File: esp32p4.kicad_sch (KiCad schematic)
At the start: 51 parts, among them U13 W25Q128JVS, U3 TLV62569DBV, U8 ESP32P4-REV0, Y3 40MHz

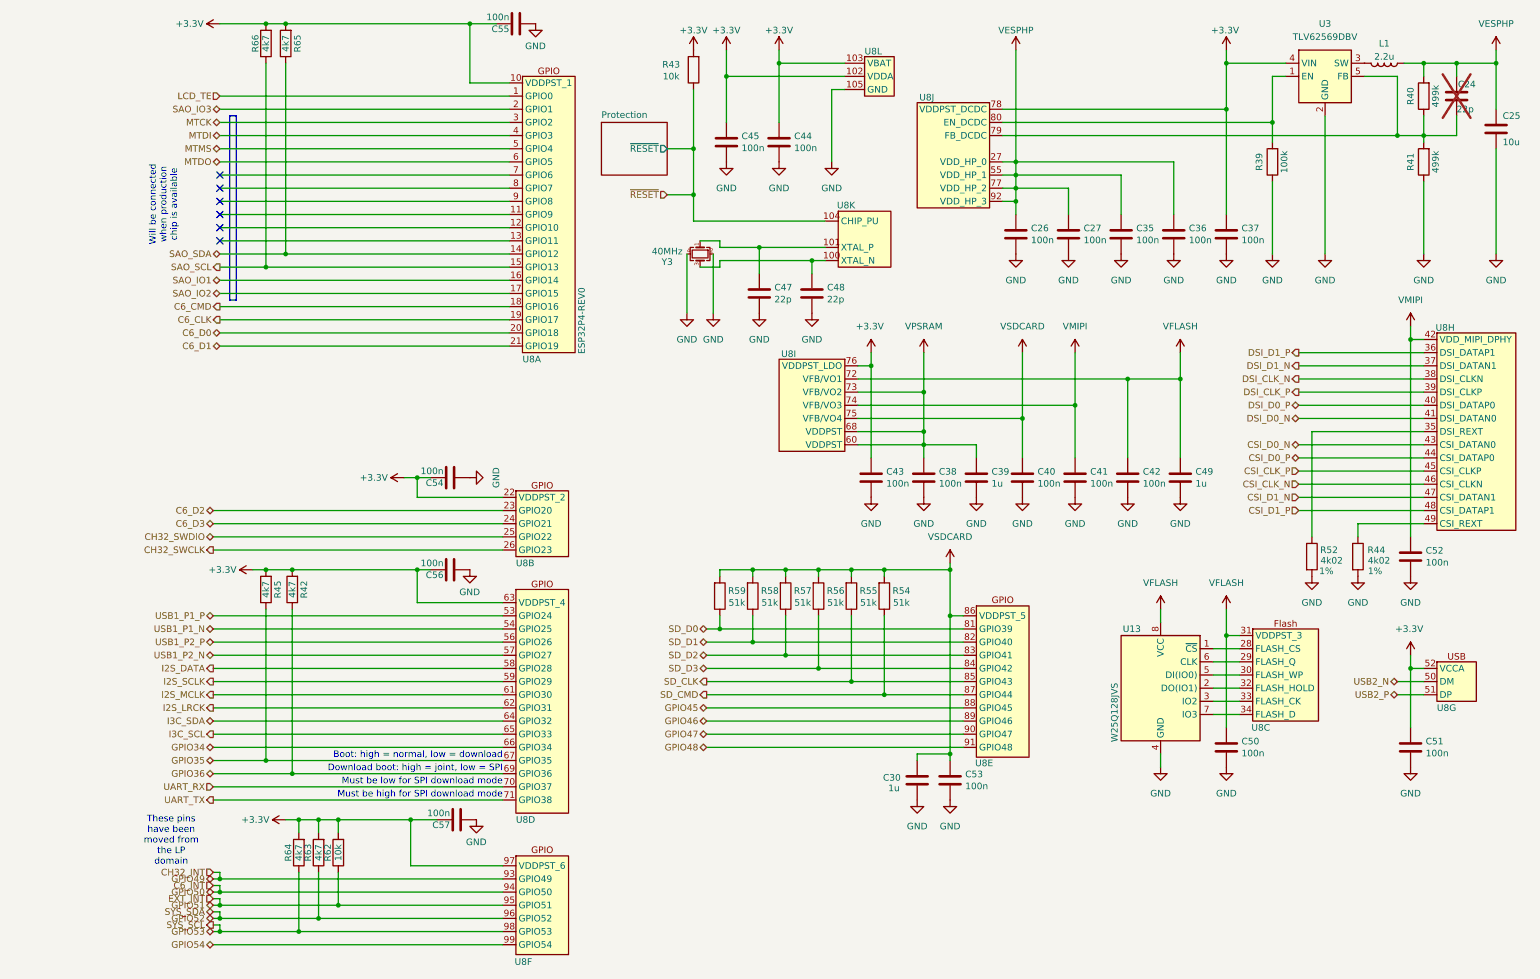
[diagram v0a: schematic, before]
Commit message: More routing, moved some more signals
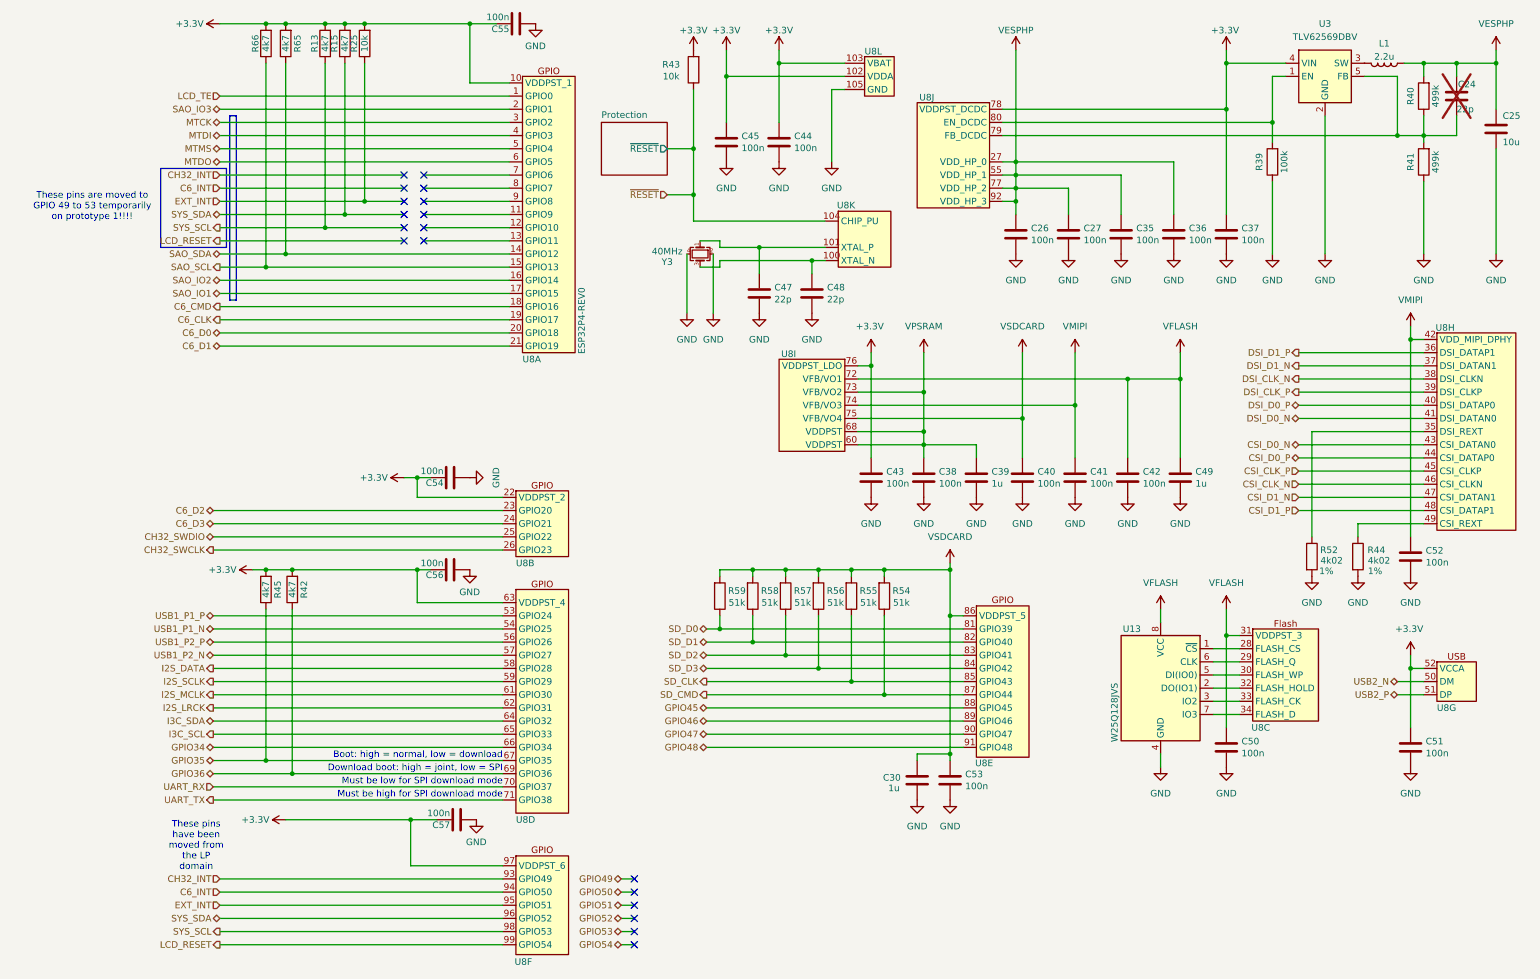
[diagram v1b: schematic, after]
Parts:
- removed R62: 10k, Resistor_SMD:R_0402_1005Metric, symbol Device:R
- removed R63, R64: 4k7, Resistor_SMD:R_0402_1005Metric, symbol Device:R
- added R13, R15: 4k7, Resistor_SMD:R_0402_1005Metric, symbol Device:R
- added R25: 10k, Resistor_SMD:R_0402_1005Metric, symbol Device:R
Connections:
- net +3.3V: now also R13.2, R15.2, R25.2
- net EXT_INT: now also R25.1
- net GPIO52: no longer U8.96 (GPIO52)
- net GPIO53: no longer U8.98 (GPIO53)
- net GPIO54: no longer U8.99 (GPIO54)
- net SAO_IO1: now also U8.17 (GPIO15); no longer U8.16 (GPIO14)
- net SAO_IO2: now also U8.16 (GPIO14); no longer U8.17 (GPIO15)
- new net LCD_RESET: U8.99 (GPIO54)
- new net SYS_SCL: R13.1, U8.98 (GPIO53)
- new net SYS_SDA: R15.1, U8.96 (GPIO52)
- no-connect marks 6 -> 18
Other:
- note added: "These pins are moved to GPIO 49 to 53 temporarily on prototype 1!!!!"
- note removed: "Will be connected when production chip is available"
